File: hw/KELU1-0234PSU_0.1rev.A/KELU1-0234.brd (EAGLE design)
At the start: 50 x 85 mm, 78 parts, among them IC1 UC3844, P1 B3B-EH-A, P2 B3B-EH-A, Q2 IRF740TO220BVH, T1 E25137

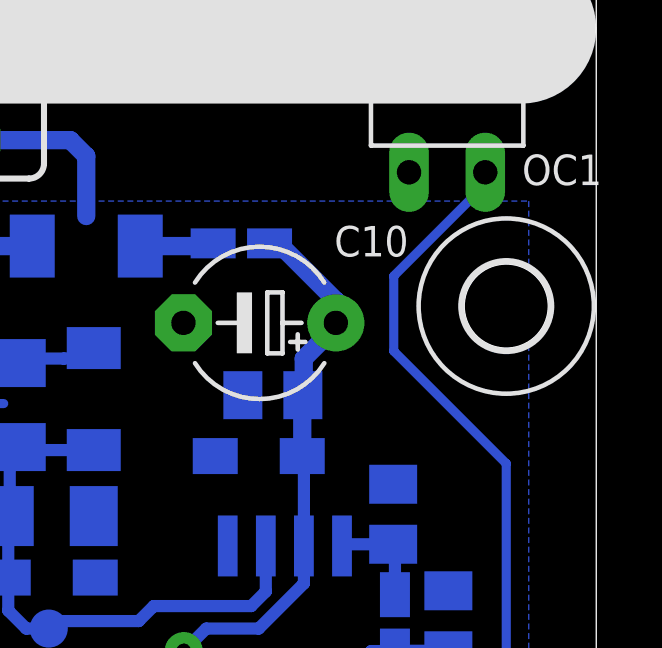
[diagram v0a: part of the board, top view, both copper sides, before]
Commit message: Add image
Add new image  pcb
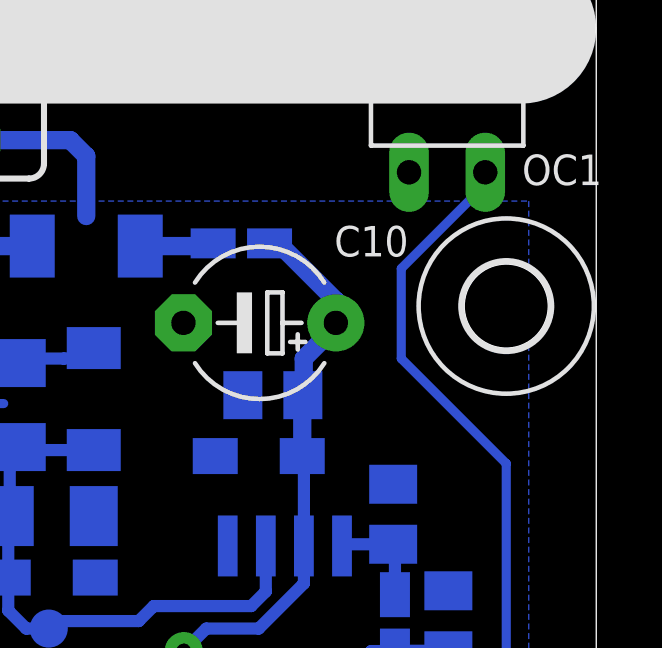
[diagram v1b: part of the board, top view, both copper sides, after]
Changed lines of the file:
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@@
 <wire x1="29" y1="37.25" x2="29" y2="43.25" width="0.6096" layer="16"/>
 <wire x1="29" y1="43.25" x2="29.5" y2="43.75" width="0.6096" layer="16"/>
-<wire x1="34.95" y1="33.15" x2="40.255" y2="32.8566" width="0" layer="19" extent="16-16"/>
 </signal>
 <signal name="N$13">
@@
 <wire x1="41.525" y1="31.475" x2="41.525" y2="32.8566" width="0.4064" layer="16"/>
 <wire x1="46.3" y1="51.46" x2="46.3" y2="51.05" width="0.3048" layer="16"/>
-<wire x1="46.3" y1="51.05" x2="43.25" y2="48" width="0.3048" layer="16"/>
-<wire x1="43.25" y1="48" x2="43.25" y2="45.5" width="0.3048" layer="16"/>
-<wire x1="43.25" y1="45.5" x2="47" y2="41.75" width="0.3048" layer="16"/>
+<wire x1="46.3" y1="51.05" x2="43.5" y2="48.25" width="0.3048" layer="16"/>
+<wire x1="43.5" y1="45.25" x2="47" y2="41.75" width="0.3048" layer="16"/>
 <wire x1="47" y1="41.75" x2="47" y2="32" width="0.3048" layer="16"/>
 <wire x1="47" y1="32" x2="44.5" y2="29.5" width="0.3048" layer="16"/>
+<wire x1="43.5" y1="48.25" x2="43.5" y2="45.25" width="0.3048" layer="16"/>
 </signal>
 <signal name="N$31">

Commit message: Revert "Update"
This reverts commit e262ecb1de31ac634c25b05378be0f730255bc1c.
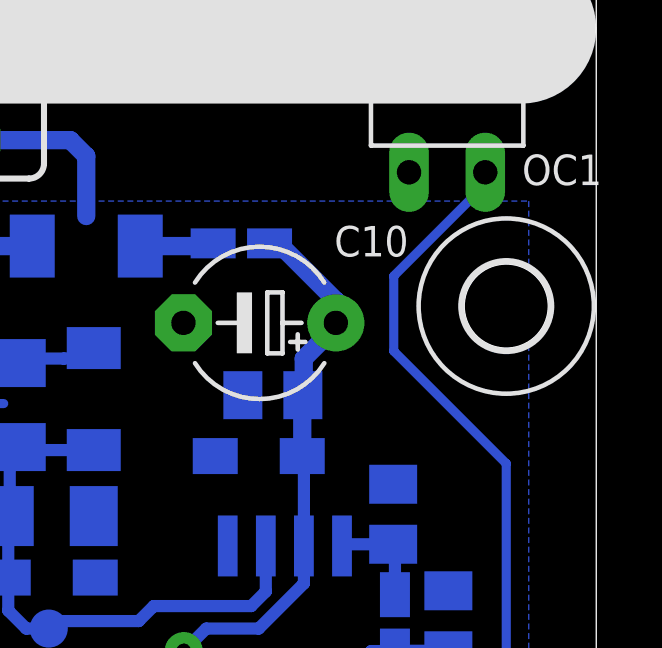
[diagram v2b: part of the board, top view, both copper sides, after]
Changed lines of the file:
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@@
 <wire x1="29" y1="37.25" x2="29" y2="43.25" width="0.6096" layer="16"/>
 <wire x1="29" y1="43.25" x2="29.5" y2="43.75" width="0.6096" layer="16"/>
+<wire x1="34.95" y1="33.15" x2="40.255" y2="32.8566" width="0" layer="19" extent="16-16"/>
 </signal>
 <signal name="N$13">
@@
 <wire x1="41.525" y1="31.475" x2="41.525" y2="32.8566" width="0.4064" layer="16"/>
 <wire x1="46.3" y1="51.46" x2="46.3" y2="51.05" width="0.3048" layer="16"/>
-<wire x1="46.3" y1="51.05" x2="43.5" y2="48.25" width="0.3048" layer="16"/>
-<wire x1="43.5" y1="45.25" x2="47" y2="41.75" width="0.3048" layer="16"/>
+<wire x1="46.3" y1="51.05" x2="43.25" y2="48" width="0.3048" layer="16"/>
+<wire x1="43.25" y1="48" x2="43.25" y2="45.5" width="0.3048" layer="16"/>
+<wire x1="43.25" y1="45.5" x2="47" y2="41.75" width="0.3048" layer="16"/>
 <wire x1="47" y1="41.75" x2="47" y2="32" width="0.3048" layer="16"/>
 <wire x1="47" y1="32" x2="44.5" y2="29.5" width="0.3048" layer="16"/>
-<wire x1="43.5" y1="48.25" x2="43.5" y2="45.25" width="0.3048" layer="16"/>
 </signal>
 <signal name="N$31">
